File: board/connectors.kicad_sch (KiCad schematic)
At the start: 8 parts, among them J3 Power, J4 LED, J5 SWD6p, J6 Connections

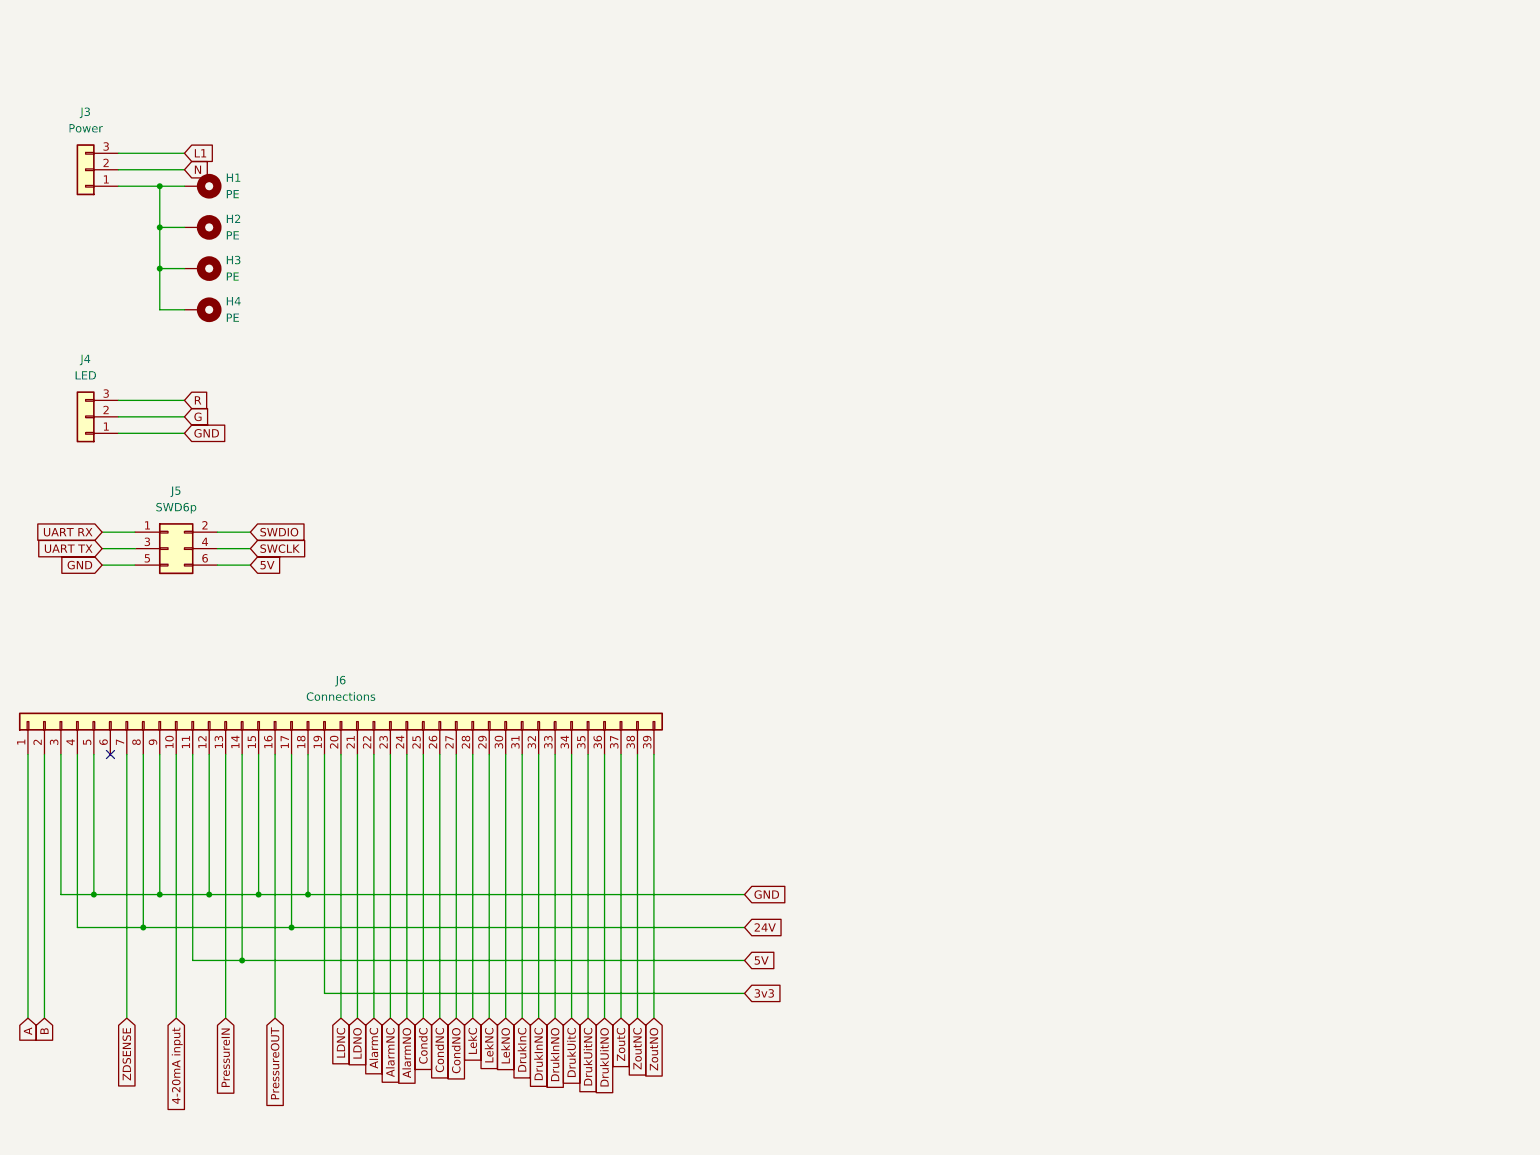
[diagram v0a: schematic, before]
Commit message: pushpushpush
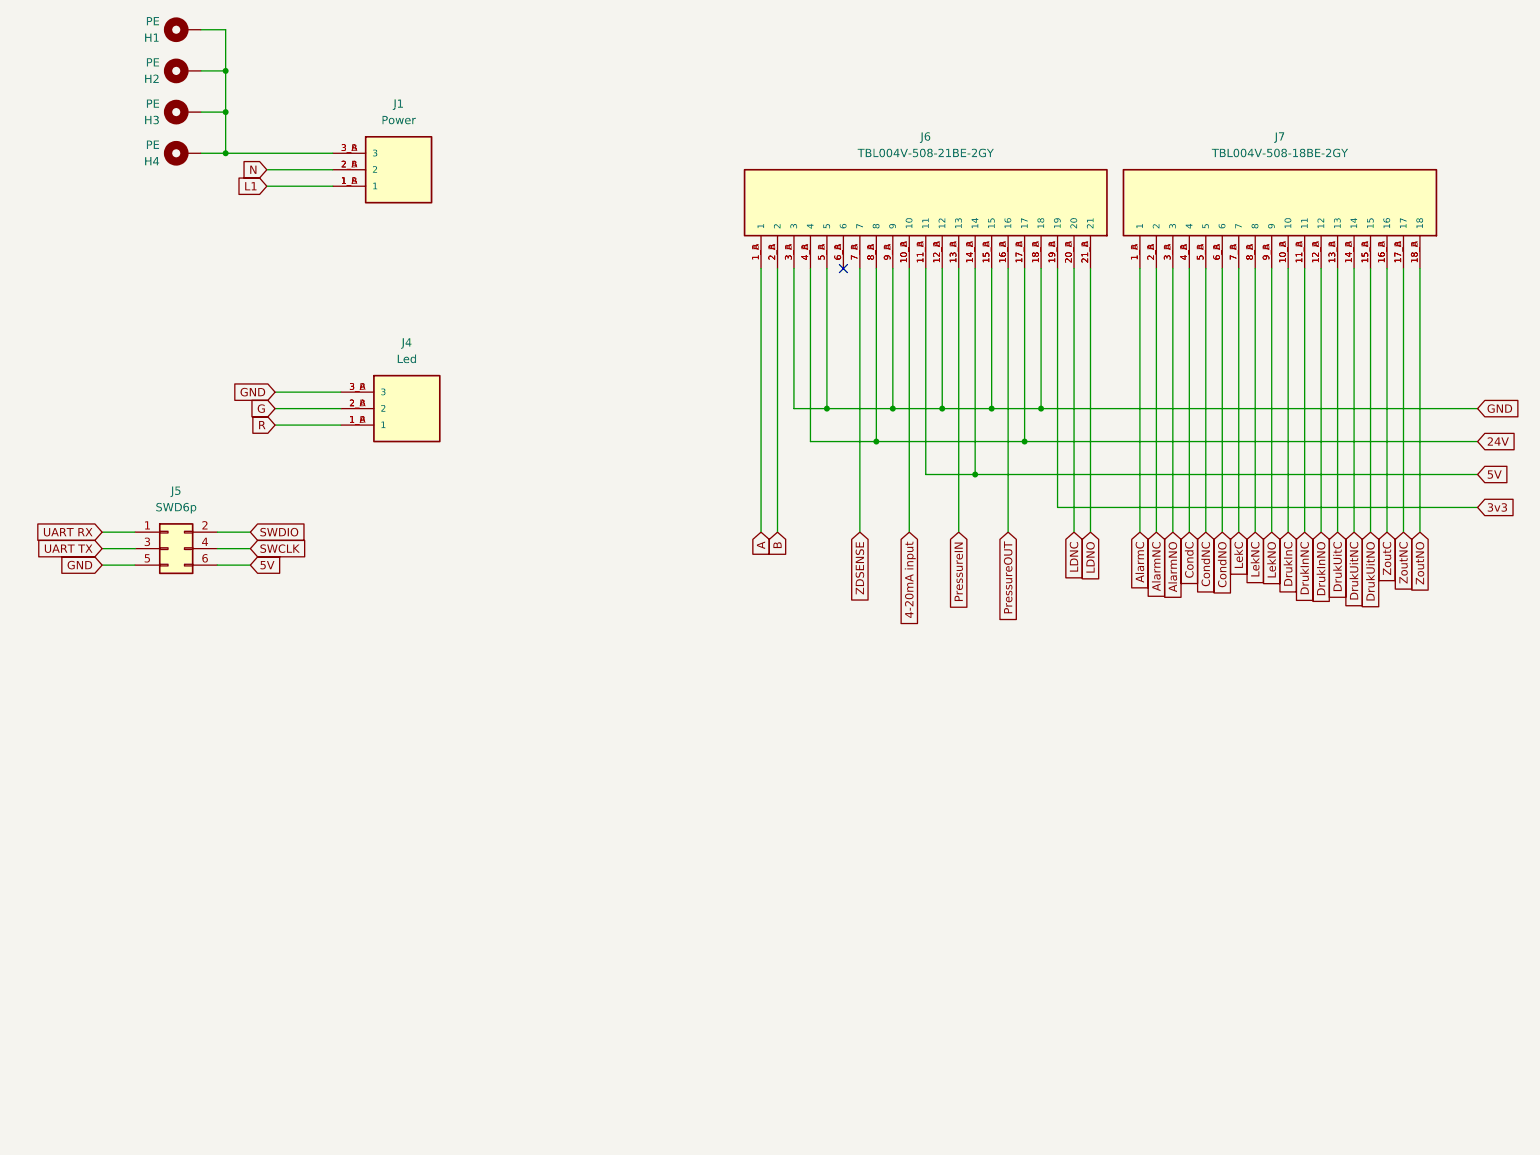
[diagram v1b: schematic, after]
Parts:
- removed J3: Power, Connector_PinHeader_2.54mm:PinHeader_1x03_P2.54mm_Vertical, symbol Connector_Generic:Conn_01x03
- removed J4: LED, Connector_PinHeader_2.54mm:PinHeader_1x03_P2.54mm_Vertical, symbol Connector_Generic:Conn_01x03
- removed J6: Connections, Connector_PinHeader_2.54mm:PinHeader_1x39_P2.54mm_Vertical, symbol Connector_Generic:Conn_01x39
- added J1: Power, kicad_libs:CUI_TBL004V-508-03BE-2GY, symbol TBL004V-508-03BE-2GY:TBL004V-508-03BE-2GY
- added J4: Led, kicad_libs:CUI_TBL004V-508-03BE-2GY, symbol TBL004V-508-03BE-2GY:TBL004V-508-03BE-2GY
- added J6: TBL004V-508-21BE-2GY, kicad_libs:CUI_TBL004V-508-21BE-2GY, symbol TBL004V-508-21BE-2GY:TBL004V-508-21BE-2GY
- added J7: TBL004V-508-18BE-2GY, kicad_libs:CUI_TBL004V-508-18BE-2GY, symbol TBL004V-508-18BE-2GY:TBL004V-508-18BE-2GY
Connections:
- net 24V: now also J6.17_A (17), J6.17_B (17), J6.4_A (4), J6.4_B (4), J6.8_A (8), J6.8_B (8)
- net 3v3: now also J6.19_A (19), J6.19_B (19)
- net 4-20mA input: now also J6.10_A (10), J6.10_B (10)
- net 5V: now also J6.11_A (11), J6.11_B (11), J6.14_A (14), J6.14_B (14)
- net A: now also J6.1_A (1), J6.1_B (1)
- net AlarmC: now also J7.1_A (1), J7.1_B (1)
- net AlarmNC: now also J7.2_A (2), J7.2_B (2)
- net AlarmNO: now also J7.3_A (3), J7.3_B (3)
- net B: now also J6.2_A (2), J6.2_B (2)
- net CondC: now also J7.4_A (4), J7.4_B (4)
- net CondNC: now also J7.5_A (5), J7.5_B (5)
- net CondNO: now also J7.6_A (6), J7.6_B (6)
- net DrukInC: now also J7.10_A (10), J7.10_B (10)
- net DrukInNC: now also J7.11_A (11), J7.11_B (11)
- net DrukInNO: now also J7.12_A (12), J7.12_B (12)
- net DrukUitC: now also J7.13_A (13), J7.13_B (13)
- net DrukUitNC: now also J7.14_A (14), J7.14_B (14)
- net DrukUitNO: now also J7.15_A (15), J7.15_B (15)
- net G: now also J4.2_A (2), J4.2_B (2)
- net GND: now also J4.3_A (3), J4.3_B (3), J6.12_A (12), J6.12_B (12), J6.15_A (15), J6.15_B (15), J6.18_A (18), J6.18_B (18), J6.3_A (3), J6.3_B (3), J6.5_A (5), J6.5_B (5), J6.9_A (9), J6.9_B (9)
- net L1: now also J1.1_A (1), J1.1_B (1)
- net LDNC: now also J6.20_A (20), J6.20_B (20)
- net LDNO: now also J6.21_A (21), J6.21_B (21)
- net LekC: now also J7.7_A (7), J7.7_B (7)
- net LekNC: now also J7.8_A (8), J7.8_B (8)
- net LekNO: now also J7.9_A (9), J7.9_B (9)
- net N: now also J1.2_A (2), J1.2_B (2)
- net PressureIN: now also J6.13_A (13), J6.13_B (13)
- net PressureOUT: now also J6.16_A (16), J6.16_B (16)
- net R: now also J4.1_A (1), J4.1_B (1)
- net ZDSENSE: now also J6.7_A (7), J6.7_B (7)
- net ZoutC: now also J7.16_A (16), J7.16_B (16)
- net ZoutNC: now also J7.17_A (17), J7.17_B (17)
- net ZoutNO: now also J7.18_A (18), J7.18_B (18)
- net at H1.1, H2.1, H3.1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: now also J1.3_A (3), J1.3_B (3)
- new net: J6.6_A (6), J6.6_B (6)
